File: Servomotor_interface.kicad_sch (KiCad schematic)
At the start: 41 parts, among them J7 JST B6B XH A, U3 VNH7070

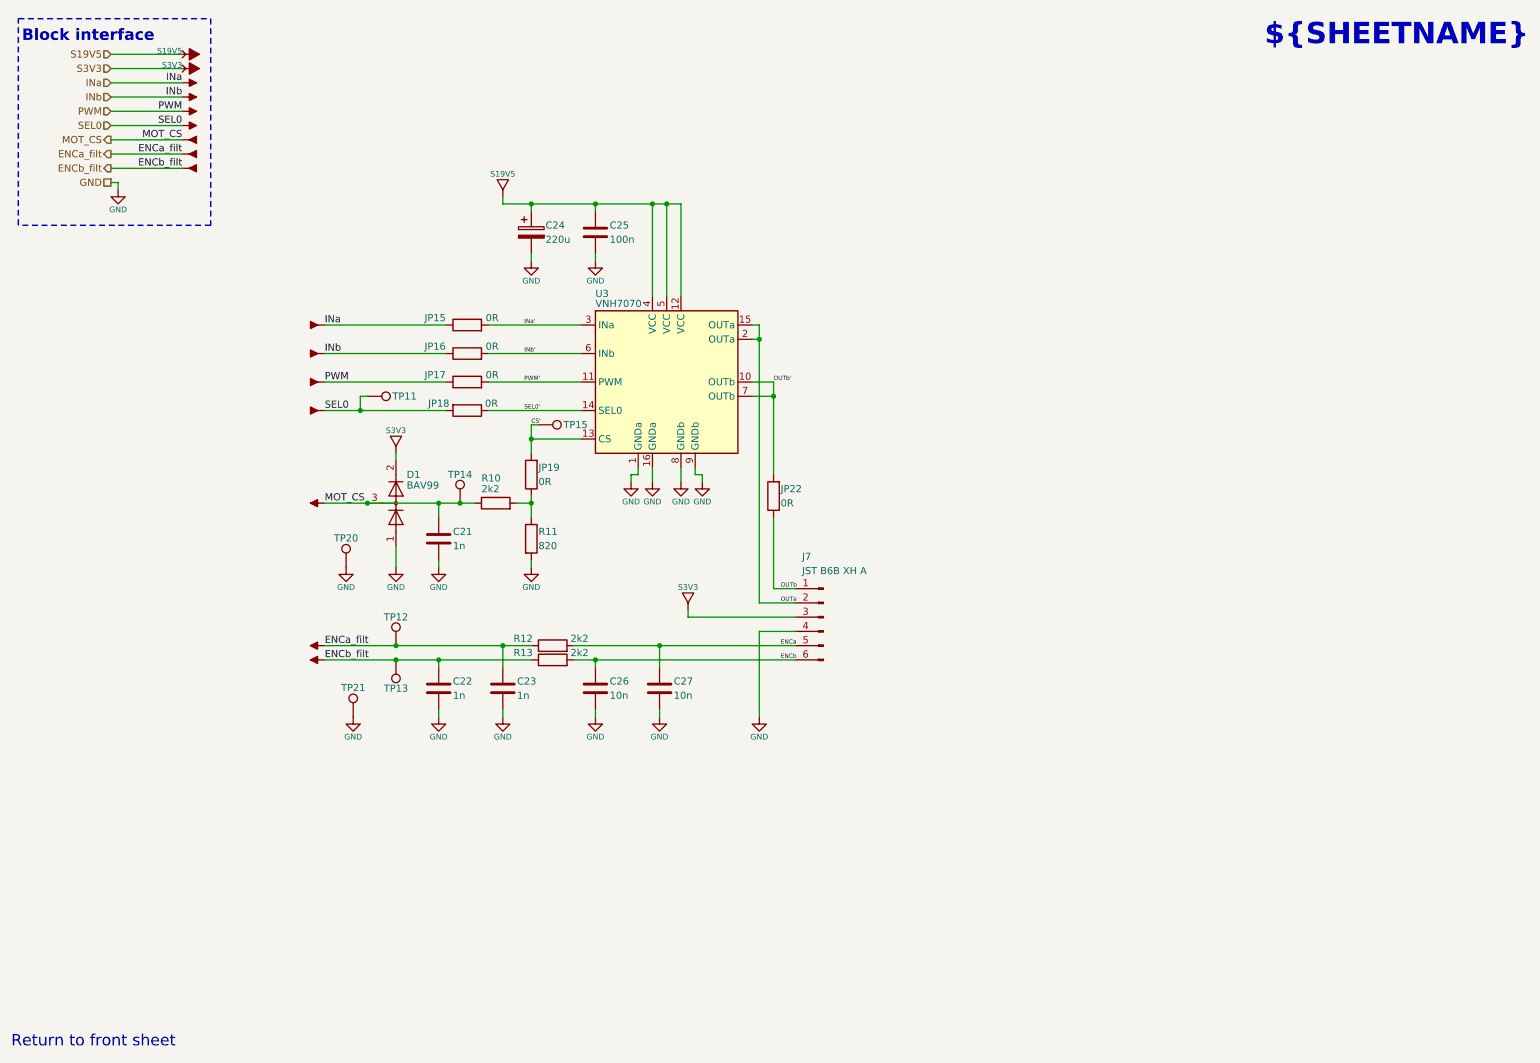
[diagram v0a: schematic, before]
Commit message: reorganised sch and pcb
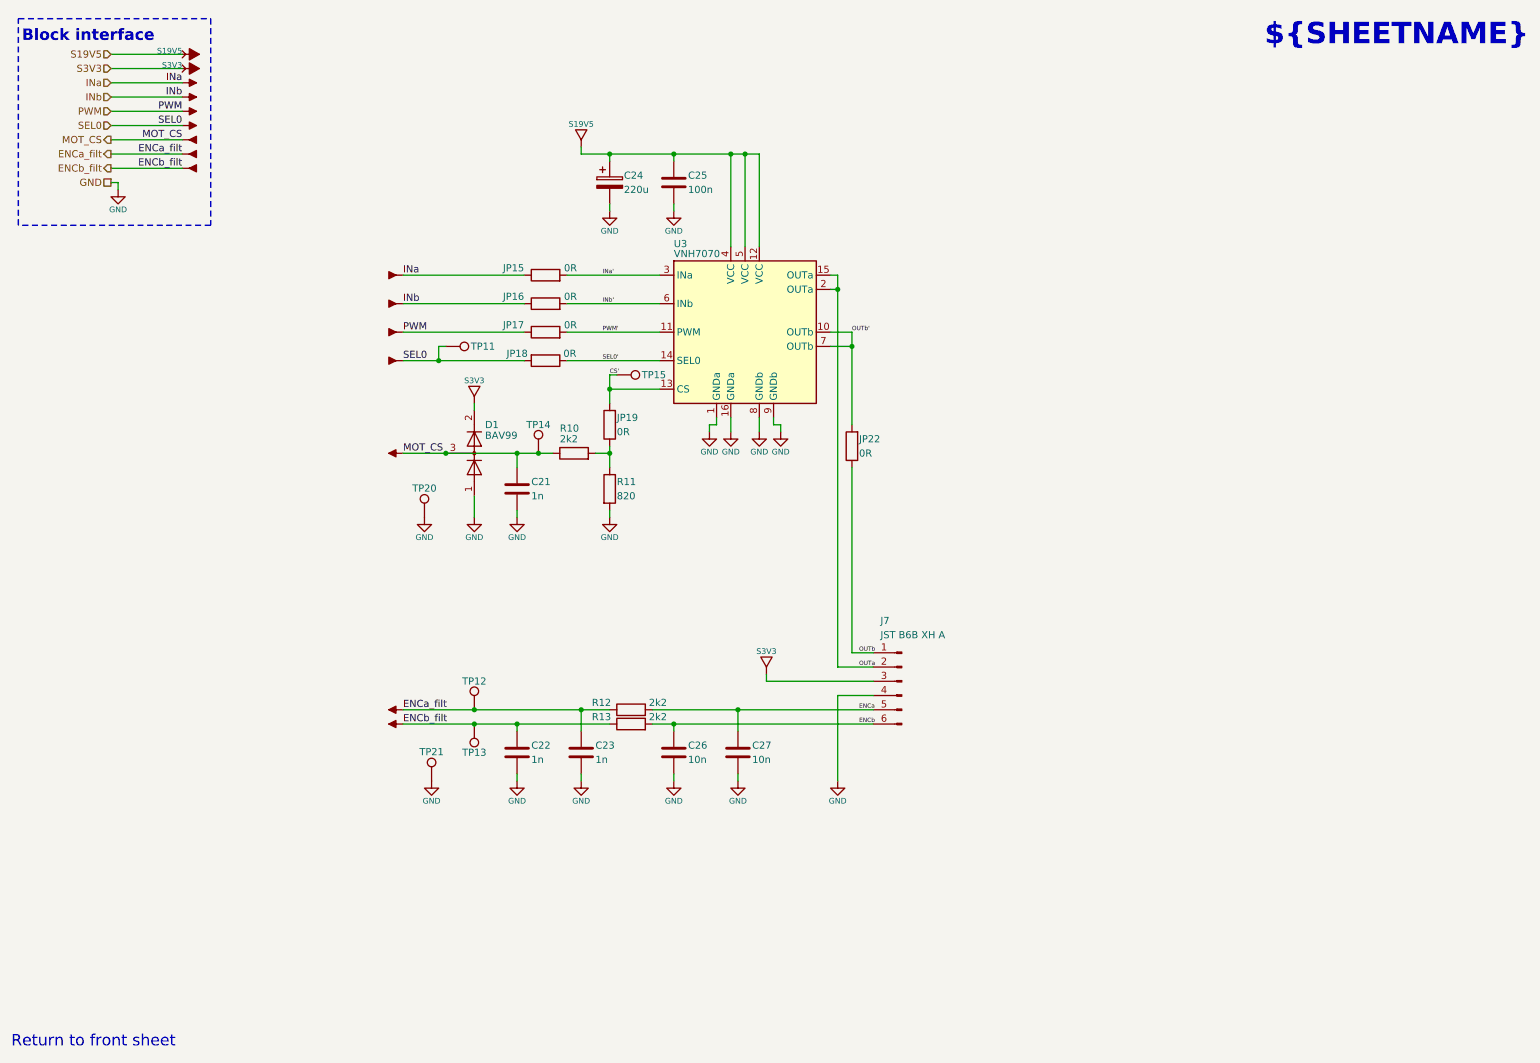
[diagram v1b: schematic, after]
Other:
- moved on the sheet: C21, C22, C23, C24, C25, C26, C27, D1, J7, JP15, JP16, JP17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
